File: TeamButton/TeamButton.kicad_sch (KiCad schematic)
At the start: 7 parts, among them J1 RJ45, SW1 10T85 Microswitch, SW2 10T85 Microswitch

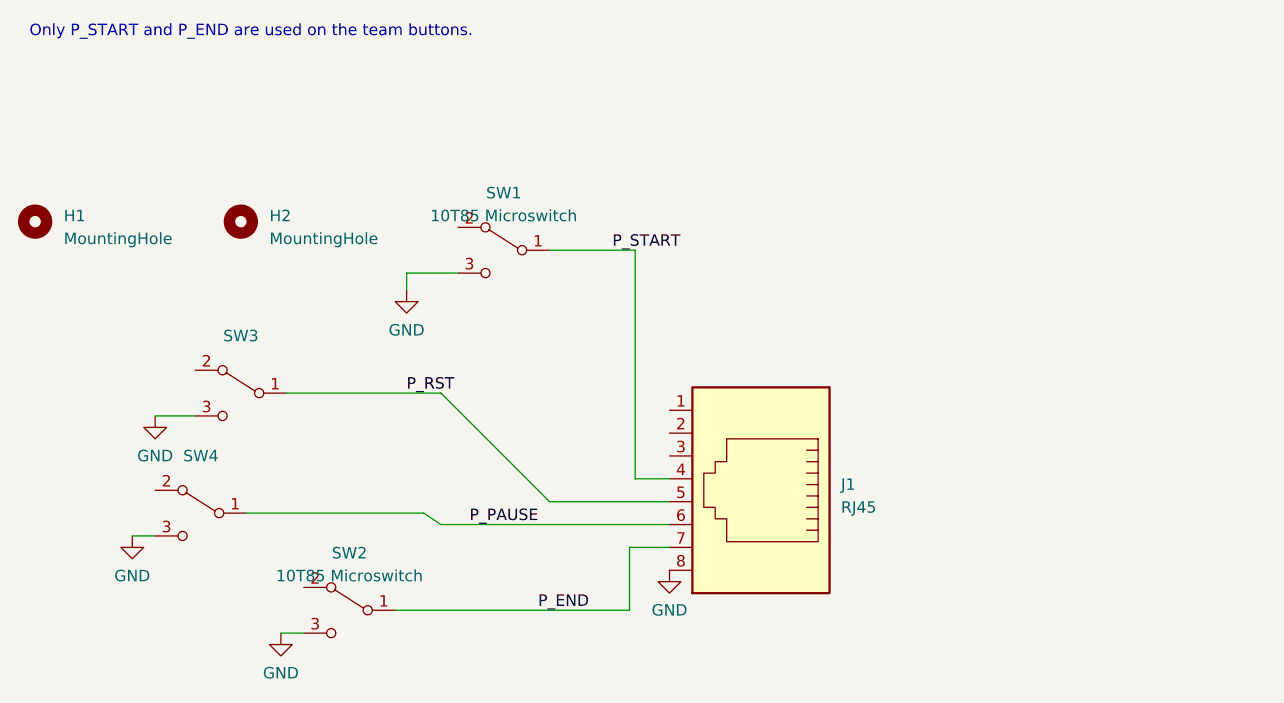
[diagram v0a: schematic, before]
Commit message: Release 7/19/23
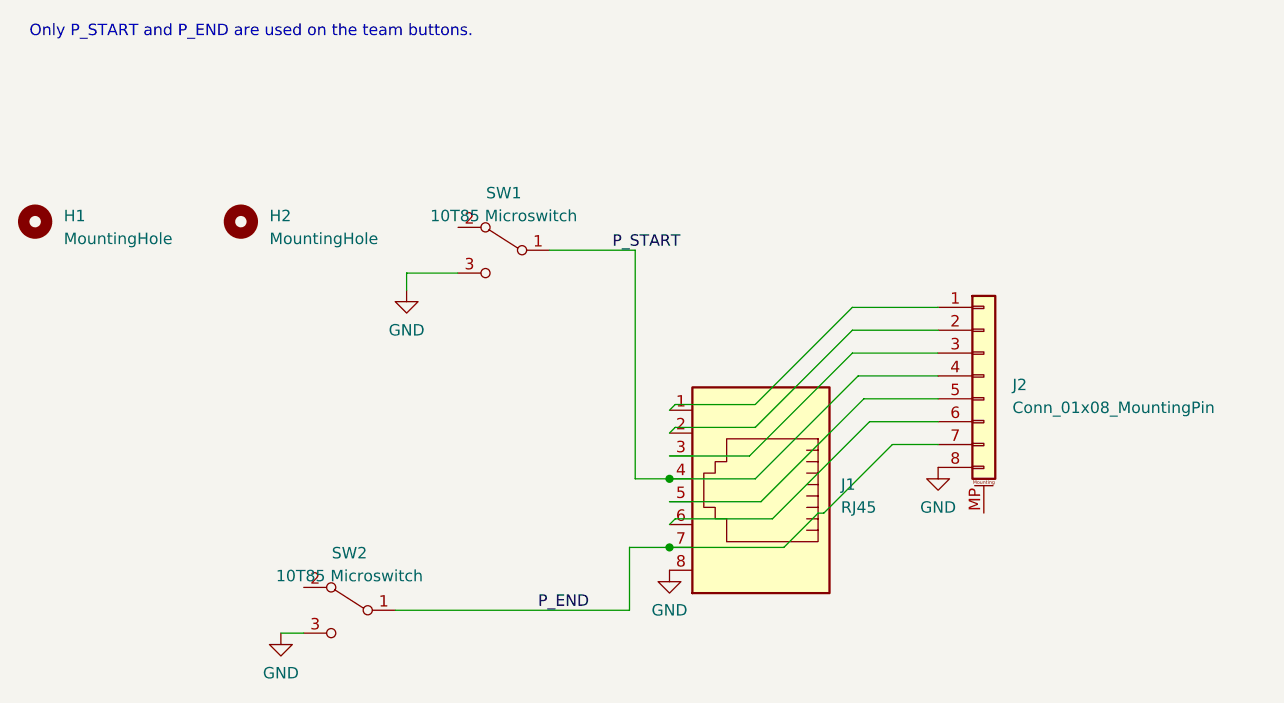
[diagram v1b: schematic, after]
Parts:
- removed SW3, SW4: (no value), Connector_PinSocket_2.00mm:PinSocket_1x03_P2.00mm_Vertical, symbol symbols:10T85 Microswitch
- added J2: Conn_01x08_MountingPin, Connector_PinSocket_2.54mm:PinSocket_1x08_P2.54mm_Horizontal, symbol Connector_Generic_MountingPin:Conn_01x08_MountingPin
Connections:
- net GND: now also J2.8 (Pin_8)
- net P_END: now also J2.7 (Pin_7)
- net P_START: now also J2.4 (Pin_4)
- net at J1.1: now also J2.1 (Pin_1)
- net at J1.2: now also J2.2 (Pin_2)
- net at J1.3: now also J2.3 (Pin_3)
- net P_PAUSE: no longer names the net of J1.6
- net P_PAUSE: now also J2.6 (Pin_6)
- net P_RST: no longer names the net of J1.5
- net P_RST: now also J2.5 (Pin_5)
